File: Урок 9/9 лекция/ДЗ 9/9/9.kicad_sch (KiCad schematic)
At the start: 25 parts, among them IC1 LM393P, SW1 SW_Push

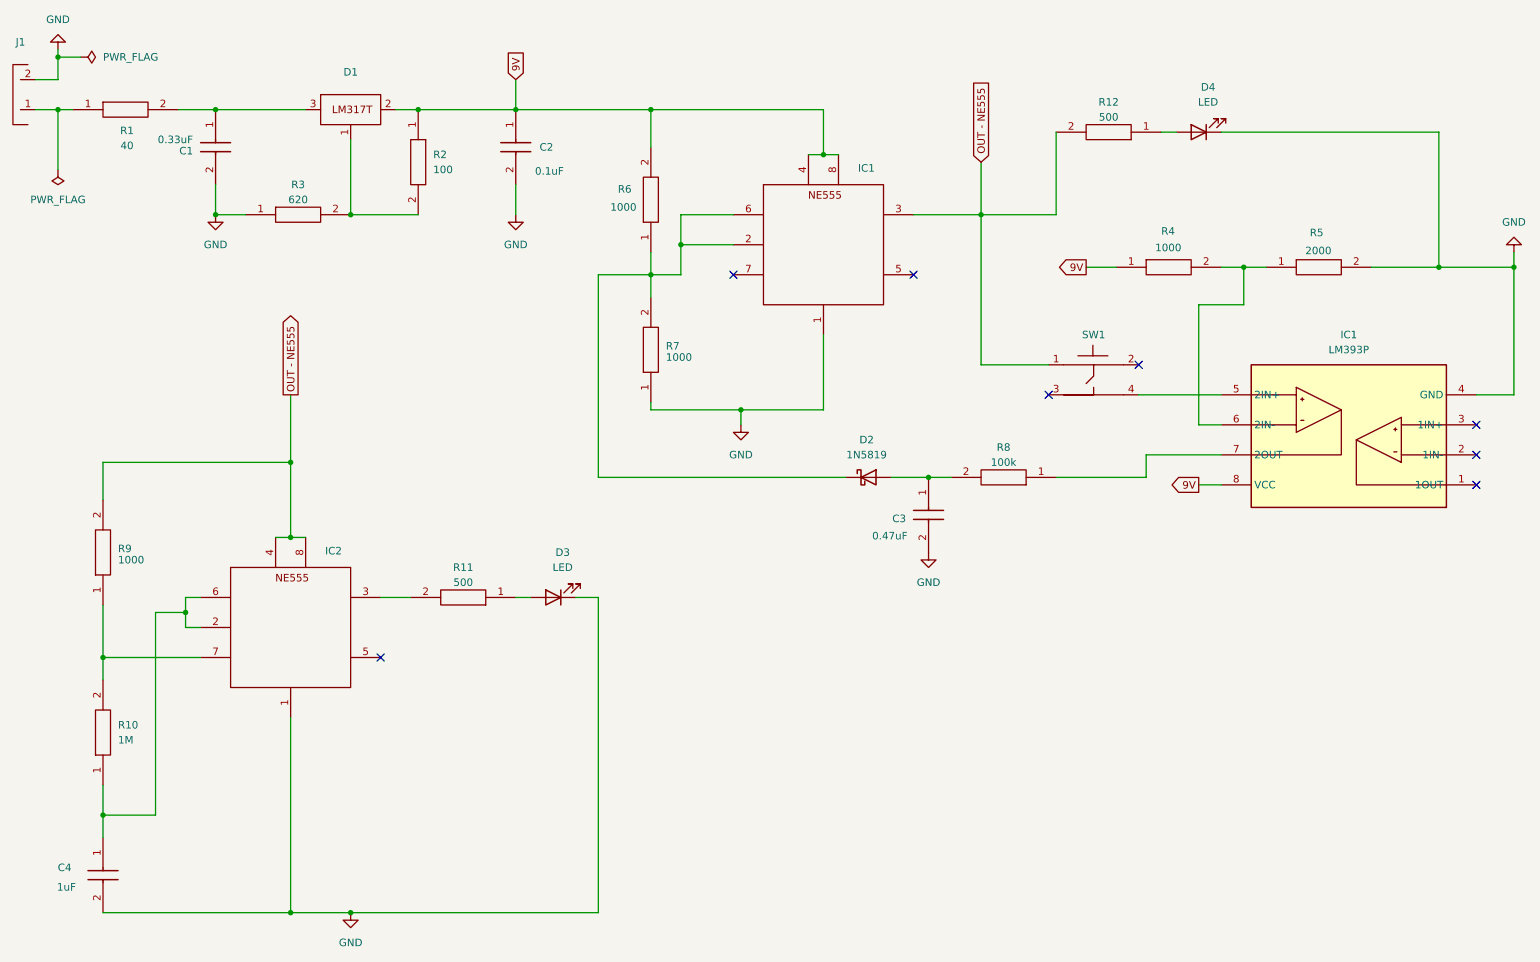
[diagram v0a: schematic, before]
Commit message: Финал
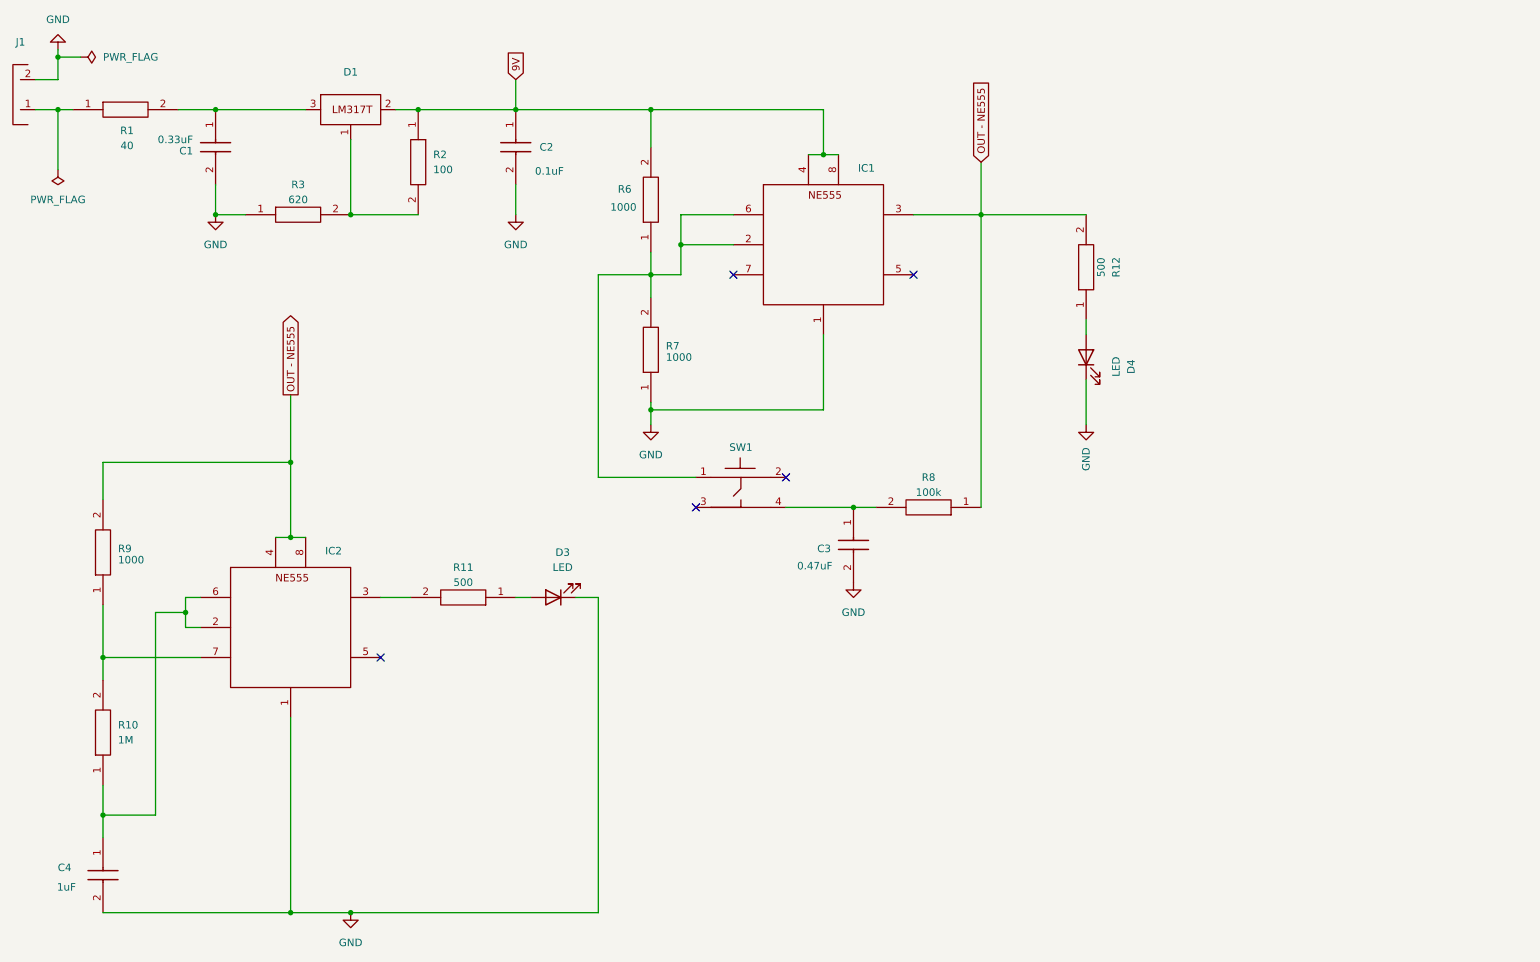
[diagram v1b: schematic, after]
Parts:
- removed D2: 1N5819, Diode_THT:D_DO-35_SOD27_P7.62mm_Horizontal, symbol Diode:1N5711
- removed IC1: LM393P, My_lib2:8-DIP, symbol My_lib2:LM393P
- removed R4: 1000, My_lib2:R axil, symbol My_lib2:R_CF100-3K3-J-TB-070-62
- removed R5: 2000, My_lib2:R axil, symbol My_lib2:R_CF100-3K3-J-TB-070-62
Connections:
- net OUT - NE555: now also R8.1; no longer SW1.1
- net at IC1.2, IC1.6, R6.1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: now also SW1.1
- net at C3.1, R8.2: now also SW1.4 (2)
- no-connect marks 8 -> 5
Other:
- moved on the sheet: C3, D4, R12, R8, SW1
